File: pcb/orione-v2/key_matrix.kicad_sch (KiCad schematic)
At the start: 124 parts, among them SW1 SW_Push, SW10 SW_Push, SW11 SW_Push, SW12 SW_Push, SW13 SW_Push, SW14 SW_Push, SW15 SW_Push, SW16 SW_Push, SW17 SW_Push, SW18 SW_Push, SW19 SW_Push, SW2 SW_Push, SW20 SW_Push, SW21 SW_Push, SW22 SW_Push, SW23 SW_Push, SW24 SW_Push, SW25 SW_Push, SW26 SW_Push, SW27 SW_Push, SW28 SW_Push, SW29 SW_Push, SW3 SW_Push, SW30 SW_Push, SW31 SW_Push, SW32 SW_Push, SW33 SW_Push, SW34 SW_Push, SW35 SW_Push, SW36 SW_Push, SW37 SW_Push, SW38 SW_Push, SW39 SW_Push, SW4 SW_Push, SW40 SW_Push, SW41 SW_Push, SW42 SW_Push, SW43 SW_Push, SW44 SW_Push, SW45 SW_Push, SW46 SW_Push, SW47 SW_Push, SW48 SW_Push, SW49 SW_Push, SW5 SW_Push, SW50 SW_Push, SW51 SW_Push, SW52 SW_Push, SW53 SW_Push, SW54 SW_Push, SW55 SW_Push, SW56 SW_Push, SW57 SW_Push, SW58 SW_Push, SW59 SW_Push, SW6 SW_Push, SW60 SW_Push, SW61 SW_Push, SW62 SW_Push, SW7 SW_Push, SW8 SW_Push, SW9 SW_Push

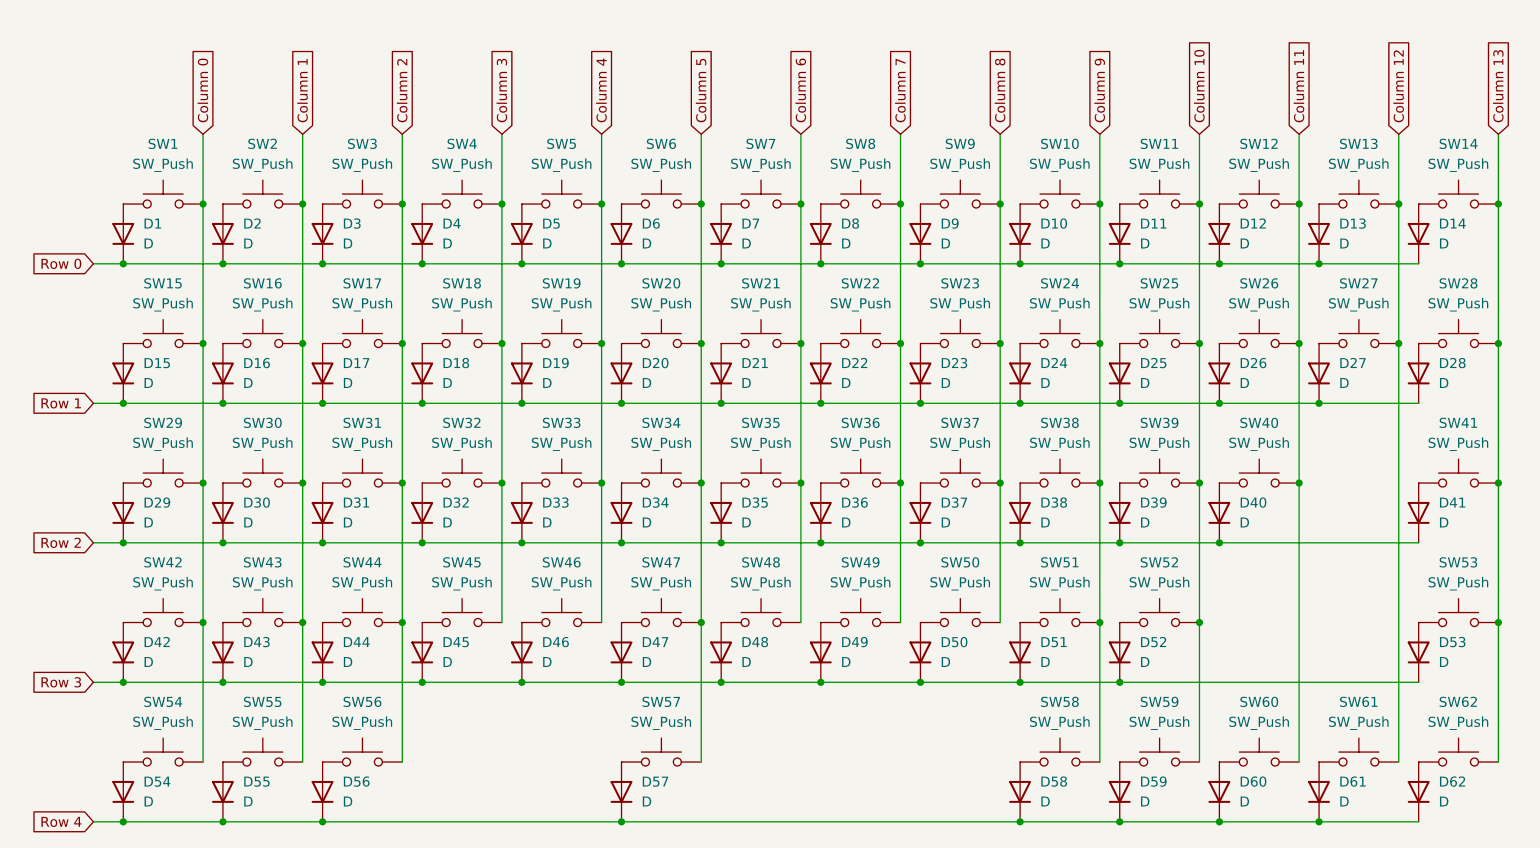
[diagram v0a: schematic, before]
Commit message: pcb
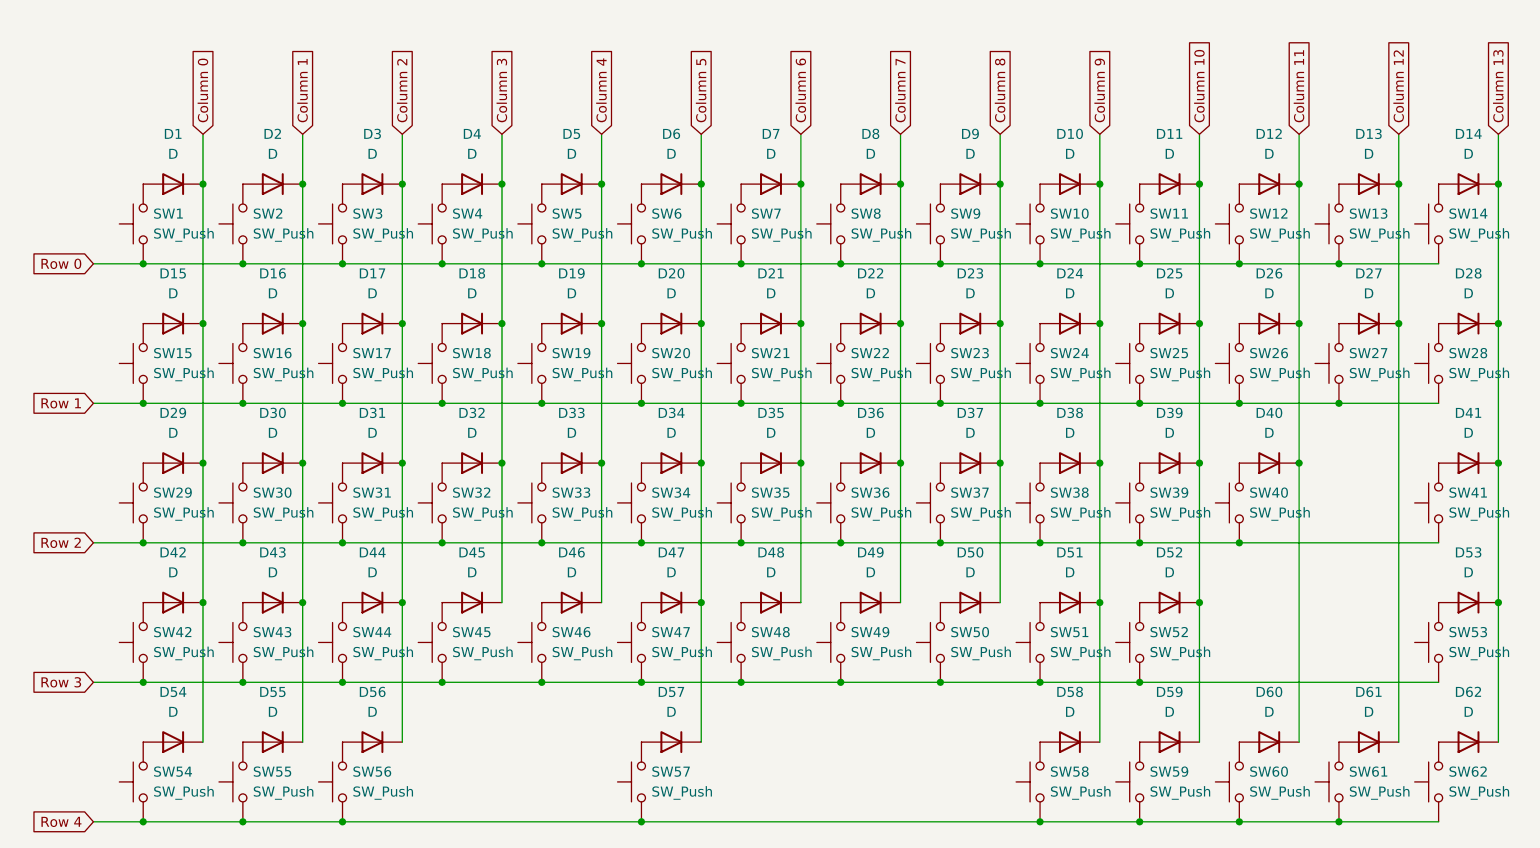
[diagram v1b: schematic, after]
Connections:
- net Column 0: now also D1.1 (K), D15.1 (K), D29.1 (K), D42.1 (K), D54.1 (K); no longer SW1.2, SW15.2, SW29.2, SW42.2, SW54.2
- net Column 1: now also D16.1 (K), D2.1 (K), D30.1 (K), D43.1 (K), D55.1 (K); no longer SW16.2, SW2.2, SW30.2, SW43.2, SW55.2
- net Column 10: now also D11.1 (K), D25.1 (K), D39.1 (K), D52.1 (K), D59.1 (K); no longer SW11.2, SW25.2, SW39.2, SW52.2, SW59.2
- net Column 11: now also D12.1 (K), D26.1 (K), D40.1 (K), D60.1 (K); no longer SW12.2, SW26.2, SW40.2, SW60.2
- net Column 12: now also D13.1 (K), D27.1 (K), D61.1 (K); no longer SW13.2, SW27.2, SW61.2
- net Column 13: now also D14.1 (K), D28.1 (K), D41.1 (K), D53.1 (K), D62.1 (K); no longer SW14.2, SW28.2, SW41.2, SW53.2, SW62.2
- net Column 2: now also D17.1 (K), D3.1 (K), D31.1 (K), D44.1 (K), D56.1 (K); no longer SW17.2, SW3.2, SW31.2, SW44.2, SW56.2
- net Column 3: now also D18.1 (K), D32.1 (K), D4.1 (K), D45.1 (K); no longer SW18.2, SW32.2, SW4.2, SW45.2
- net Column 4: now also D19.1 (K), D33.1 (K), D46.1 (K), D5.1 (K); no longer SW19.2, SW33.2, SW46.2, SW5.2
- net Column 5: now also D20.1 (K), D34.1 (K), D47.1 (K), D57.1 (K), D6.1 (K); no longer SW20.2, SW34.2, SW47.2, SW57.2, SW6.2
- net Column 6: now also D21.1 (K), D35.1 (K), D48.1 (K), D7.1 (K); no longer SW21.2, SW35.2, SW48.2, SW7.2
- net Column 7: now also D22.1 (K), D36.1 (K), D49.1 (K), D8.1 (K); no longer SW22.2, SW36.2, SW49.2, SW8.2
- net Column 8: now also D23.1 (K), D37.1 (K), D50.1 (K), D9.1 (K); no longer SW23.2, SW37.2, SW50.2, SW9.2
- net Column 9: now also D10.1 (K), D24.1 (K), D38.1 (K), D51.1 (K), D58.1 (K); no longer SW10.2, SW24.2, SW38.2, SW51.2, SW58.2
- net Row 0: now also SW1.1, SW10.1, SW11.1, SW12.1, SW13.1, SW14.1, SW2.1, SW3.1, SW4.1, SW5.1, SW6.1, SW7.1, SW8.1, SW9.1; no longer D1.1 (K), D10.1 (K), D11.1 (K), D12.1 (K), D13.1 (K), D14.1 (K), D2.1 (K), D3.1 (K), D4.1 (K), D5.1 (K), D6.1 (K), D7.1 (K), D8.1 (K), D9.1 (K)
- net Row 1: now also SW15.1, SW16.1, SW17.1, SW18.1, SW19.1, SW20.1, SW21.1, SW22.1, SW23.1, SW24.1, SW25.1, SW26.1, SW27.1, SW28.1; no longer D15.1 (K), D16.1 (K), D17.1 (K), D18.1 (K), D19.1 (K), D20.1 (K), D21.1 (K), D22.1 (K), D23.1 (K), D24.1 (K), D25.1 (K), D26.1 (K), D27.1 (K), D28.1 (K)
- net Row 2: now also SW29.1, SW30.1, SW31.1, SW32.1, SW33.1, SW34.1, SW35.1, SW36.1, SW37.1, SW38.1, SW39.1, SW40.1, SW41.1; no longer D29.1 (K), D30.1 (K), D31.1 (K), D32.1 (K), D33.1 (K), D34.1 (K), D35.1 (K), D36.1 (K), D37.1 (K), D38.1 (K), D39.1 (K), D40.1 (K), D41.1 (K)
- net Row 3: now also SW42.1, SW43.1, SW44.1, SW45.1, SW46.1, SW47.1, SW48.1, SW49.1, SW50.1, SW51.1, SW52.1, SW53.1; no longer D42.1 (K), D43.1 (K), D44.1 (K), D45.1 (K), D46.1 (K), D47.1 (K), D48.1 (K), D49.1 (K), D50.1 (K), D51.1 (K), D52.1 (K), D53.1 (K)
- net Row 4: now also SW54.1, SW55.1, SW56.1, SW57.1, SW58.1, SW59.1, SW60.1, SW61.1, SW62.1; no longer D54.1 (K), D55.1 (K), D56.1 (K), D57.1 (K), D58.1 (K), D59.1 (K), D60.1 (K), D61.1 (K), D62.1 (K)
- net at D6.2 (A): now also SW6.2; no longer SW6.1
- net at D8.2 (A): now also SW8.2; no longer SW8.1
- net at D23.2 (A): now also SW23.2; no longer SW23.1
- net at D56.2 (A): now also SW56.2; no longer SW56.1
- net at D7.2 (A): now also SW7.2; no longer SW7.1
- net at D26.2 (A): now also SW26.2; no longer SW26.1
- net at D30.2 (A): now also SW30.2; no longer SW30.1
- net at D46.2 (A): now also SW46.2; no longer SW46.1
- net at D54.2 (A): now also SW54.2; no longer SW54.1
- net at D28.2 (A): now also SW28.2; no longer SW28.1
- net at D12.2 (A): now also SW12.2; no longer SW12.1
- net at D48.2 (A): now also SW48.2; no longer SW48.1
- net at D5.2 (A): now also SW5.2; no longer SW5.1
- net at D51.2 (A): now also SW51.2; no longer SW51.1
- net at D21.2 (A): now also SW21.2; no longer SW21.1
- net at D3.2 (A): now also SW3.2; no longer SW3.1
- net at D45.2 (A): now also SW45.2; no longer SW45.1
- net at D43.2 (A): now also SW43.2; no longer SW43.1
- net at D11.2 (A): now also SW11.2; no longer SW11.1
- net at D10.2 (A): now also SW10.2; no longer SW10.1
- net at D34.2 (A): now also SW34.2; no longer SW34.1
- net at D58.2 (A): now also SW58.2; no longer SW58.1
- net at D49.2 (A): now also SW49.2; no longer SW49.1
- net at D13.2 (A): now also SW13.2; no longer SW13.1
- net at D40.2 (A): now also SW40.2; no longer SW40.1
- net at D9.2 (A): now also SW9.2; no longer SW9.1
- net at D33.2 (A): now also SW33.2; no longer SW33.1
- net at D24.2 (A): now also SW24.2; no longer SW24.1
- net at D27.2 (A): now also SW27.2; no longer SW27.1
- net at D36.2 (A): now also SW36.2; no longer SW36.1
- net at D53.2 (A): now also SW53.2; no longer SW53.1
- net at D57.2 (A): now also SW57.2; no longer SW57.1
- net at D15.2 (A): now also SW15.2; no longer SW15.1
- net at D17.2 (A): now also SW17.2; no longer SW17.1
- net at D4.2 (A): now also SW4.2; no longer SW4.1
- net at D44.2 (A): now also SW44.2; no longer SW44.1
- net at D42.2 (A): now also SW42.2; no longer SW42.1
- net at D50.2 (A): now also SW50.2; no longer SW50.1
- net at D41.2 (A): now also SW41.2; no longer SW41.1
- net at D22.2 (A): now also SW22.2; no longer SW22.1
- net at D60.2 (A): now also SW60.2; no longer SW60.1
- net at D31.2 (A): now also SW31.2; no longer SW31.1
- net at D55.2 (A): now also SW55.2; no longer SW55.1
- net at D1.2 (A): now also SW1.2; no longer SW1.1
- net at D59.2 (A): now also SW59.2; no longer SW59.1
- net at D38.2 (A): now also SW38.2; no longer SW38.1
- net at D37.2 (A): now also SW37.2; no longer SW37.1
- net at D29.2 (A): now also SW29.2; no longer SW29.1
- net at D61.2 (A): now also SW61.2; no longer SW61.1
- net at D20.2 (A): now also SW20.2; no longer SW20.1
- net at D16.2 (A): now also SW16.2; no longer SW16.1
- net at D35.2 (A): now also SW35.2; no longer SW35.1
- net at D32.2 (A): now also SW32.2; no longer SW32.1
- net at D62.2 (A): now also SW62.2; no longer SW62.1
- net at D52.2 (A): now also SW52.2; no longer SW52.1
- net at D18.2 (A): now also SW18.2; no longer SW18.1
- net at D47.2 (A): now also SW47.2; no longer SW47.1
- net at D25.2 (A): now also SW25.2; no longer SW25.1
- net at D14.2 (A): now also SW14.2; no longer SW14.1
- net at D39.2 (A): now also SW39.2; no longer SW39.1
- net at D19.2 (A): now also SW19.2; no longer SW19.1
- net at D2.2 (A): now also SW2.2; no longer SW2.1
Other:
- moved on the sheet: D1, SW1
